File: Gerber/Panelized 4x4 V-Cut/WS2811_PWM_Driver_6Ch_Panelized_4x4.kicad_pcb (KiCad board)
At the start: 2 copper layers, 100 x 100 mm, 656 parts, among them P1 Com, P2 PWM, P3 HS/LS, P4 HS/LS, P5 GND, P6 DIFIN, P7 DIFOUT, Q1 MMBT4401, Q2 MMBT4401, Q3 MMBT4401, Q4 MMBT4401, Q5 MMBT4401, Q6 MMBT4401, U1 SP485, U2 WS2811, U3 WS2811, U4 SP485

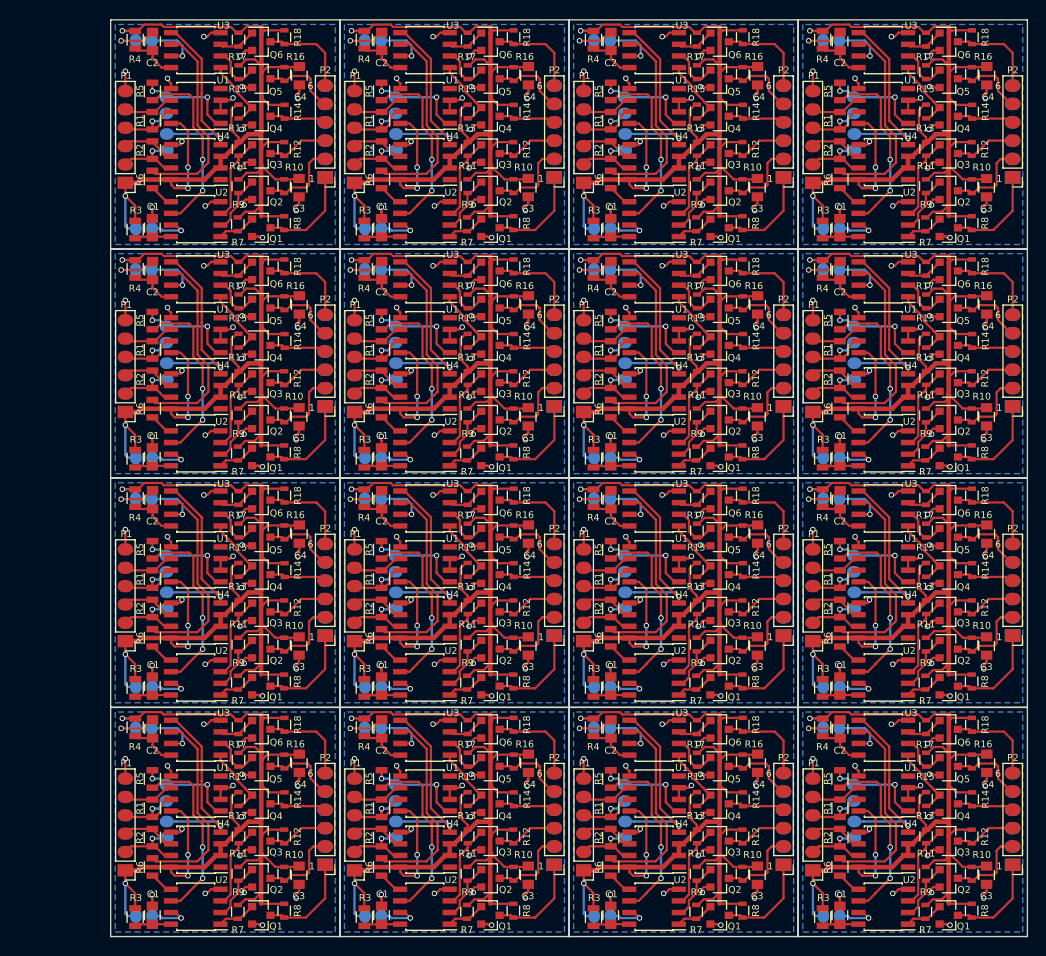
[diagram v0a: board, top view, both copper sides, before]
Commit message: Gerber Updates
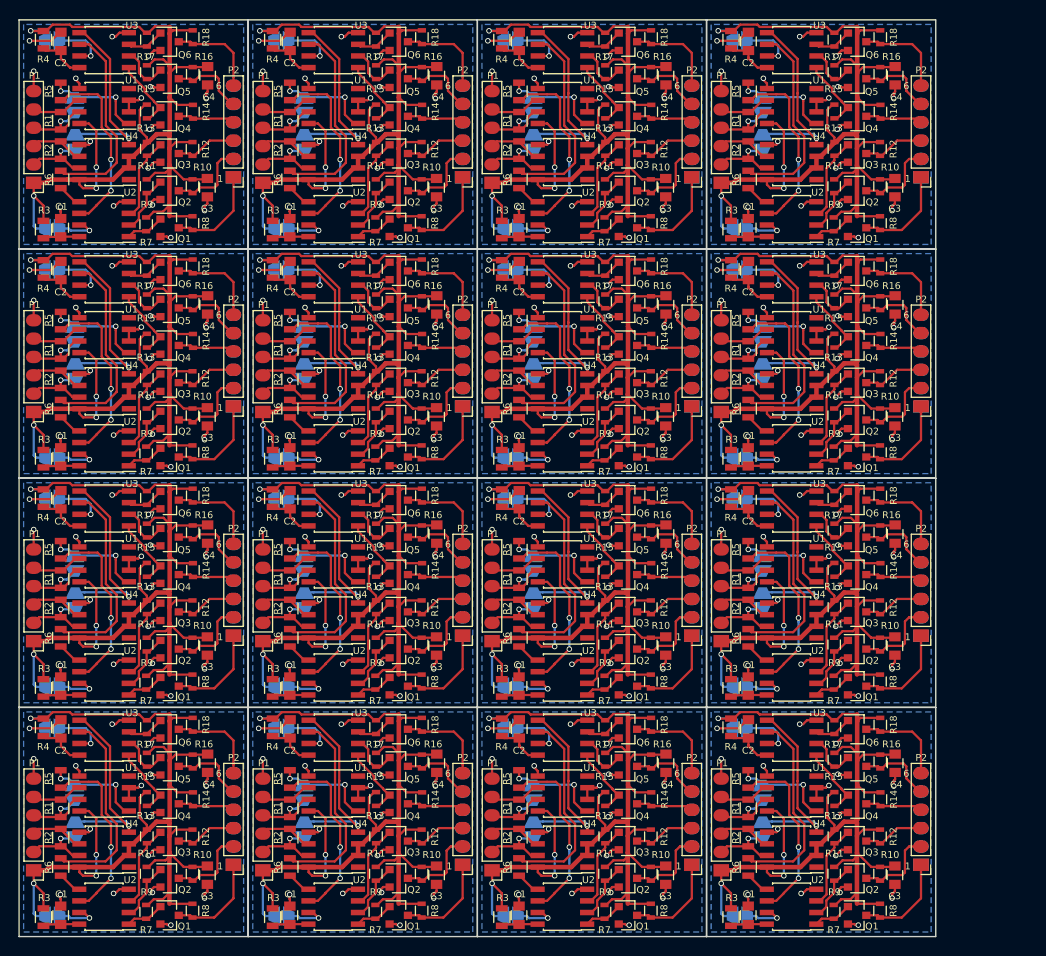
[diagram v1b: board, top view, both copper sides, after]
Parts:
- removed the C1 at (154.5, 147.7)
- removed the C1 at (129.5, 97.7)
- removed the C1 at (104.5, 97.7)
- removed the C1 at (179.5, 97.7)
- removed the C1 at (179.5, 72.7)
- removed the C1 at (154.5, 72.7)
- removed the C1 at (129.5, 72.7)
- removed the C1 at (129.5, 147.7)
- removed the C1 at (104.5, 147.7)
- removed the C1 at (179.5, 147.7)
- removed the C1 at (154.5, 122.7)
- removed the C1 at (129.5, 122.7)
- removed the C1 at (104.5, 122.7)
- removed the C1 at (179.5, 122.7)
- removed the C1 at (154.5, 97.7)
- removed the C2 at (154.6, 127.3)
- removed the C2 at (129.6, 77.3)
- removed the C2 at (104.6, 77.3)
- removed the C2 at (179.6, 77.3)
- removed the C2 at (179.6, 52.3)
- removed the C2 at (154.6, 52.3)
- removed the C2 at (129.6, 52.3)
- removed the C2 at (129.6, 127.3)
- removed the C2 at (104.6, 127.3)
- removed the C2 at (179.6, 127.3)
- removed the C2 at (154.6, 102.3)
- removed the C2 at (129.6, 102.3)
- removed the C2 at (104.6, 102.3)
- removed the C2 at (179.6, 102.3)
- removed the C2 at (154.6, 77.3)
- removed the C3 at (170.5, 143.3)
- removed the C3 at (145.5, 93.3)
- removed the C3 at (120.5, 93.3)
- removed the C3 at (195.5, 93.3)
- removed the C3 at (195.5, 68.3)
- removed the C3 at (170.5, 68.3)
- removed the C3 at (145.5, 68.3)
- removed the C3 at (145.5, 143.3)
- removed the C3 at (120.5, 143.3)
- removed the C3 at (195.5, 143.3)
- removed the C3 at (170.5, 118.3)
- removed the C3 at (145.5, 118.3)
- removed the C3 at (120.5, 118.3)
- removed the C3 at (195.5, 118.3)
- removed the C3 at (170.5, 93.3)
- removed the C4 at (170.6, 131.1)
- removed the C4 at (145.6, 81.1)
- removed the C4 at (120.6, 81.1)
- removed the C4 at (195.6, 81.1)
- removed the C4 at (195.6, 56.1)
- removed the C4 at (170.6, 56.1)
- removed the C4 at (145.6, 56.1)
- removed the C4 at (145.6, 131.1)
- removed the C4 at (120.6, 131.1)
- removed the C4 at (195.6, 131.1)
- removed the C4 at (170.6, 106.1)
- removed the C4 at (145.6, 106.1)
- removed the C4 at (120.6, 106.1)
- removed the C4 at (195.6, 106.1)
- removed the C4 at (170.6, 81.1)
- removed the P1 at (151.6, 142.8)
- removed the P1 at (126.6, 92.8)
- removed the P1 at (101.6, 92.8)
- removed the P1 at (176.6, 92.8)
- removed the P1 at (176.6, 67.8)
- removed the P1 at (151.6, 67.8)
- removed the P1 at (126.6, 67.8)
- removed the P1 at (126.6, 142.8)
- removed the P1 at (101.6, 142.8)
- removed the P1 at (176.6, 142.8)
- removed the P1 at (151.6, 117.8)
- removed the P1 at (126.6, 117.8)
- removed the P1 at (101.6, 117.8)
- removed the P1 at (176.6, 117.8)
- removed the P1 at (151.6, 92.8)
- removed the P2 at (148.4, 142.2)
- removed the P2 at (123.4, 92.2)
- removed the P2 at (173.4, 92.2)
- removed the P2 at (198.4, 92.2)
- removed the P2 at (198.4, 67.2)
- removed the P2 at (173.4, 67.2)
- removed the P2 at (148.4, 67.2)
- removed the P2 at (123.4, 142.2)
- removed the P2 at (173.4, 142.2)
- removed the P2 at (198.4, 142.2)
- removed the P2 at (148.4, 117.2)
- removed the P2 at (123.4, 117.2)
- removed the P2 at (173.4, 117.2)
- removed the P2 at (198.4, 117.2)
- removed the P2 at (148.4, 92.2)
- removed the P3 at (153.6, 147.8)
- removed the P3 at (178.6, 97.8)
- removed the P3 at (103.6, 97.8)
- removed the P3 at (128.6, 97.8)
- removed the P3 at (178.6, 72.8)
- removed the P3 at (153.6, 72.8)
- removed the P3 at (128.6, 72.8)
- removed the P3 at (178.6, 147.8)
- removed the P3 at (103.6, 147.8)
- removed the P3 at (128.6, 147.8)
- removed the P3 at (153.6, 122.8)
- removed the P3 at (178.6, 122.8)
- removed the P3 at (103.6, 122.8)
- removed the P3 at (128.6, 122.8)
- removed the P3 at (153.6, 97.8)
- removed the P4 at (153.6, 127.3)
- removed the P4 at (178.6, 77.3)
- removed the P4 at (103.6, 77.3)
- removed the P4 at (128.6, 77.3)
- removed the P4 at (178.6, 52.3)
- removed the P4 at (153.6, 52.3)
- removed the P4 at (128.6, 52.3)
- removed the P4 at (178.6, 127.3)
- removed the P4 at (103.6, 127.3)
- removed the P4 at (128.6, 127.3)
- removed the P4 at (153.6, 102.3)
- removed the P4 at (178.6, 102.3)
- removed the P4 at (103.6, 102.3)
- removed the P4 at (128.6, 102.3)
- removed the P4 at (153.6, 77.3)
- removed the P5 at (198.4, 142.2)
- removed the P5 at (148.4, 92.2)
- removed the P5 at (173.4, 92.2)
- removed the P5 at (123.4, 92.2)
- removed the P5 at (198.4, 67.2)
- removed the P5 at (173.4, 67.2)
- removed the P5 at (148.4, 67.2)
- removed the P5 at (148.4, 142.2)
- removed the P5 at (173.4, 142.2)
- removed the P5 at (123.4, 142.2)
- removed the P5 at (198.4, 117.2)
- removed the P5 at (148.4, 117.2)
- removed the P5 at (173.4, 117.2)
- removed the P5 at (123.4, 117.2)
- removed the P5 at (198.4, 92.2)
- removed the P6 at (181.1, 134.3)
- removed the P6 at (156.1, 84.3)
- removed the P6 at (106.1, 84.3)
- removed the P6 at (131.1, 84.3)
- removed the P6 at (181.1, 59.3)
- removed the P6 at (156.1, 59.3)
- removed the P6 at (131.1, 59.3)
- removed the P6 at (156.1, 134.3)
- removed the P6 at (106.1, 134.3)
- removed the P6 at (131.1, 134.3)
- removed the P6 at (181.1, 109.3)
- removed the P6 at (156.1, 109.3)
- removed the P6 at (106.1, 109.3)
- removed the P6 at (131.1, 109.3)
- removed the P6 at (181.1, 84.3)
- removed the P7 at (181.1, 138.3)
- removed the P7 at (156.1, 88.3)
- removed the P7 at (106.1, 88.3)
- removed the P7 at (131.1, 88.3)
- removed the P7 at (181.1, 63.3)
- removed the P7 at (156.1, 63.3)
- removed the P7 at (131.1, 63.3)
- removed the P7 at (156.1, 138.3)
- removed the P7 at (106.1, 138.3)
- removed the P7 at (131.1, 138.3)
- removed the P7 at (181.1, 113.3)
- removed the P7 at (156.1, 113.3)
- removed the P7 at (106.1, 113.3)
- removed the P7 at (131.1, 113.3)
- removed the P7 at (181.1, 88.3)
- removed the Q1 at (166.4, 147.7)
- removed the Q1 at (141.4, 97.7)
- removed the Q1 at (116.4, 97.7)
- removed the Q1 at (191.4, 97.7)
- removed the Q1 at (191.4, 72.7)
- removed the Q1 at (166.4, 72.7)
- removed the Q1 at (141.4, 72.7)
- removed the Q1 at (141.4, 147.7)
- removed the Q1 at (116.4, 147.7)
- removed the Q1 at (191.4, 147.7)
- removed the Q1 at (166.4, 122.7)
- removed the Q1 at (141.4, 122.7)
- removed the Q1 at (116.4, 122.7)
- removed the Q1 at (191.4, 122.7)
- removed the Q1 at (166.4, 97.7)
- removed the Q2 at (166.4, 143.6)
- removed the Q2 at (141.4, 93.6)
- removed the Q2 at (116.4, 93.6)
- removed the Q2 at (191.4, 93.6)
- removed the Q2 at (191.4, 68.6)
- removed the Q2 at (166.4, 68.6)
- removed the Q2 at (141.4, 68.6)
- removed the Q2 at (141.4, 143.6)
- removed the Q2 at (116.4, 143.6)
- removed the Q2 at (191.4, 143.6)
- removed the Q2 at (166.4, 118.6)
- removed the Q2 at (141.4, 118.6)
- removed the Q2 at (116.4, 118.6)
- removed the Q2 at (191.4, 118.6)
- removed the Q2 at (166.4, 93.6)
- removed the Q3 at (166.4, 139.6)
- removed the Q3 at (141.4, 89.6)
- removed the Q3 at (116.4, 89.6)
- removed the Q3 at (191.4, 89.6)
- removed the Q3 at (191.4, 64.6)
- removed the Q3 at (166.4, 64.6)
- removed the Q3 at (141.4, 64.6)
- removed the Q3 at (141.4, 139.6)
- removed the Q3 at (116.4, 139.6)
- removed the Q3 at (191.4, 139.6)
- removed the Q3 at (166.4, 114.6)
- removed the Q3 at (141.4, 114.6)
- removed the Q3 at (116.4, 114.6)
- removed the Q3 at (191.4, 114.6)
- removed the Q3 at (166.4, 89.6)
- removed the Q4 at (166.4, 135.5)
- removed the Q4 at (141.4, 85.5)
- removed the Q4 at (116.4, 85.5)
- removed the Q4 at (191.4, 85.5)
- removed the Q4 at (191.4, 60.5)
- removed the Q4 at (166.4, 60.5)
- removed the Q4 at (141.4, 60.5)
- removed the Q4 at (141.4, 135.5)
- removed the Q4 at (116.4, 135.5)
- removed the Q4 at (191.4, 135.5)
- removed the Q4 at (166.4, 110.5)
- removed the Q4 at (141.4, 110.5)
- removed the Q4 at (116.4, 110.5)
- removed the Q4 at (191.4, 110.5)
- removed the Q4 at (166.4, 85.5)
- removed the Q5 at (166.4, 131.4)
- removed the Q5 at (141.4, 81.4)
- removed the Q5 at (116.4, 81.4)
- removed the Q5 at (191.4, 81.4)
- removed the Q5 at (191.4, 56.4)
- removed the Q5 at (166.4, 56.4)
- removed the Q5 at (141.4, 56.4)
- removed the Q5 at (141.4, 131.4)
- removed the Q5 at (116.4, 131.4)
- removed the Q5 at (191.4, 131.4)
- removed the Q5 at (166.4, 106.4)
- removed the Q5 at (141.4, 106.4)
- removed the Q5 at (116.4, 106.4)
- removed the Q5 at (191.4, 106.4)
- removed the Q5 at (166.4, 81.4)
- removed the Q6 at (166.4, 127.4)
- removed the Q6 at (141.4, 77.4)
- removed the Q6 at (116.4, 77.4)
- removed the Q6 at (191.4, 77.4)
- removed the Q6 at (191.4, 52.4)
- removed the Q6 at (166.4, 52.4)
- removed the Q6 at (141.4, 52.4)
- removed the Q6 at (141.4, 127.4)
- removed the Q6 at (116.4, 127.4)
- removed the Q6 at (191.4, 127.4)
- removed the Q6 at (166.4, 102.4)
- removed the Q6 at (141.4, 102.4)
- removed the Q6 at (116.4, 102.4)
- removed the Q6 at (191.4, 102.4)
- removed the Q6 at (166.4, 77.4)
- removed the R1 at (154.5, 136.0)
- removed the R1 at (129.5, 86.0)
- removed the R1 at (104.5, 86.0)
- removed the R1 at (179.5, 86.0)
- removed the R1 at (179.5, 61.0)
- removed the R1 at (154.5, 61.0)
- removed the R1 at (129.5, 61.0)
- removed the R1 at (129.5, 136.0)
- removed the R1 at (104.5, 136.0)
- removed the R1 at (179.5, 136.0)
- removed the R1 at (154.5, 111.0)
- removed the R1 at (129.5, 111.0)
- removed the R1 at (104.5, 111.0)
- removed the R1 at (179.5, 111.0)
- removed the R1 at (154.5, 86.0)
- removed the R10 at (168.9, 143.1)
- removed the R10 at (143.9, 93.1)
- removed the R10 at (118.9, 93.1)
- removed the R10 at (193.9, 93.1)
- removed the R10 at (193.9, 68.1)
- removed the R10 at (168.9, 68.1)
- removed the R10 at (143.9, 68.1)
- removed the R10 at (143.9, 143.1)
- removed the R10 at (118.9, 143.1)
- removed the R10 at (193.9, 143.1)
- removed the R10 at (168.9, 118.1)
- removed the R10 at (143.9, 118.1)
- removed the R10 at (118.9, 118.1)
- removed the R10 at (193.9, 118.1)
- removed the R10 at (168.9, 93.1)
- removed the R11 at (163.9, 139.1)
- removed the R11 at (138.9, 89.1)
- removed the R11 at (113.9, 89.1)
- removed the R11 at (188.9, 89.1)
- removed the R11 at (188.9, 64.1)
- removed the R11 at (163.9, 64.1)
- removed the R11 at (138.9, 64.1)
- removed the R11 at (138.9, 139.1)
- removed the R11 at (113.9, 139.1)
- removed the R11 at (188.9, 139.1)
- removed the R11 at (163.9, 114.1)
- removed the R11 at (138.9, 114.1)
- removed the R11 at (113.9, 114.1)
- removed the R11 at (188.9, 114.1)
- removed the R11 at (163.9, 89.1)
- removed the R12 at (168.9, 139.1)
- removed the R12 at (143.9, 89.1)
- removed the R12 at (118.9, 89.1)
- removed the R12 at (193.9, 89.1)
- removed the R12 at (193.9, 64.1)
- removed the R12 at (168.9, 64.1)
- removed the R12 at (143.9, 64.1)
- removed the R12 at (143.9, 139.1)
- removed the R12 at (118.9, 139.1)
- removed the R12 at (193.9, 139.1)
- removed the R12 at (168.9, 114.1)
- removed the R12 at (143.9, 114.1)
- removed the R12 at (118.9, 114.1)
- removed the R12 at (193.9, 114.1)
- removed the R12 at (168.9, 89.1)
- removed the R13 at (163.9, 135.0)
- removed the R13 at (138.9, 85.0)
- removed the R13 at (113.9, 85.0)
- removed the R13 at (188.9, 85.0)
- removed the R13 at (188.9, 60.0)
- removed the R13 at (163.9, 60.0)
- removed the R13 at (138.9, 60.0)
- removed the R13 at (138.9, 135.0)
- removed the R13 at (113.9, 135.0)
- removed the R13 at (188.9, 135.0)
- removed the R13 at (163.9, 110.0)
- removed the R13 at (138.9, 110.0)
- removed the R13 at (113.9, 110.0)
- removed the R13 at (188.9, 110.0)
- removed the R13 at (163.9, 85.0)
- removed the R14 at (169.0, 135.0)
- removed the R14 at (144.0, 85.0)
- removed the R14 at (119.0, 85.0)
- removed the R14 at (194.0, 85.0)
- removed the R14 at (194.0, 60.0)
- removed the R14 at (169.0, 60.0)
- removed the R14 at (144.0, 60.0)
- removed the R14 at (144.0, 135.0)
- removed the R14 at (119.0, 135.0)
- removed the R14 at (194.0, 135.0)
- removed the R14 at (169.0, 110.0)
- removed the R14 at (144.0, 110.0)
- removed the R14 at (119.0, 110.0)
- removed the R14 at (194.0, 110.0)
- removed the R14 at (169.0, 85.0)
- removed the R15 at (163.9, 130.7)
- removed the R15 at (138.9, 80.7)
- removed the R15 at (113.9, 80.7)
- removed the R15 at (188.9, 80.7)
- removed the R15 at (188.9, 55.7)
- removed the R15 at (163.9, 55.7)
- removed the R15 at (138.9, 55.7)
- removed the R15 at (138.9, 130.7)
- removed the R15 at (113.9, 130.7)
- removed the R15 at (188.9, 130.7)
- removed the R15 at (163.9, 105.7)
- removed the R15 at (138.9, 105.7)
- removed the R15 at (113.9, 105.7)
- removed the R15 at (188.9, 105.7)
- removed the R15 at (163.9, 80.7)
- removed the R16 at (168.9, 130.9)
- removed the R16 at (143.9, 80.9)
- removed the R16 at (118.9, 80.9)
- removed the R16 at (193.9, 80.9)
- removed the R16 at (193.9, 55.9)
- removed the R16 at (168.9, 55.9)
- removed the R16 at (143.9, 55.9)
- removed the R16 at (143.9, 130.9)
- removed the R16 at (118.9, 130.9)
- removed the R16 at (193.9, 130.9)
- removed the R16 at (168.9, 105.9)
- removed the R16 at (143.9, 105.9)
- removed the R16 at (118.9, 105.9)
- removed the R16 at (193.9, 105.9)
- removed the R16 at (168.9, 80.9)
- removed the R17 at (163.9, 127.2)
- removed the R17 at (138.9, 77.2)
- removed the R17 at (113.9, 77.2)
- removed the R17 at (188.9, 77.2)
- removed the R17 at (188.9, 52.2)
- removed the R17 at (163.9, 52.2)
- removed the R17 at (138.9, 52.2)
- removed the R17 at (138.9, 127.2)
- removed the R17 at (113.9, 127.2)
- removed the R17 at (188.9, 127.2)
- removed the R17 at (163.9, 102.2)
- removed the R17 at (138.9, 102.2)
- removed the R17 at (113.9, 102.2)
- removed the R17 at (188.9, 102.2)
- removed the R17 at (163.9, 77.2)
- removed the R18 at (168.9, 126.9)
- removed the R18 at (143.9, 76.9)
- removed the R18 at (118.9, 76.9)
- removed the R18 at (193.9, 76.9)
- removed the R18 at (193.9, 51.9)
- removed the R18 at (168.9, 51.9)
- removed the R18 at (143.9, 51.9)
- removed the R18 at (143.9, 126.9)
- removed the R18 at (118.9, 126.9)
- removed the R18 at (193.9, 126.9)
- removed the R18 at (168.9, 101.9)
- removed the R18 at (143.9, 101.9)
- removed the R18 at (118.9, 101.9)
- removed the R18 at (193.9, 101.9)
- removed the R18 at (168.9, 76.9)
- removed the R2 at (154.5, 139.2)
- removed the R2 at (129.5, 89.2)
- removed the R2 at (104.5, 89.2)
- removed the R2 at (179.5, 89.2)
- removed the R2 at (179.5, 64.2)
- removed the R2 at (154.5, 64.2)
- removed the R2 at (129.5, 64.2)
- removed the R2 at (129.5, 139.2)
- removed the R2 at (104.5, 139.2)
- removed the R2 at (179.5, 139.2)
- removed the R2 at (154.5, 114.2)
- removed the R2 at (129.5, 114.2)
- removed the R2 at (104.5, 114.2)
- removed the R2 at (179.5, 114.2)
- removed the R2 at (154.5, 89.2)
- removed the R3 at (152.7, 147.9)
- removed the R3 at (127.7, 97.9)
- removed the R3 at (102.7, 97.9)
- removed the R3 at (177.7, 97.9)
- removed the R3 at (177.7, 72.9)
- removed the R3 at (152.7, 72.9)
- removed the R3 at (127.7, 72.9)
- removed the R3 at (127.7, 147.9)
- removed the R3 at (102.7, 147.9)
- removed the R3 at (177.7, 147.9)
- removed the R3 at (152.7, 122.9)
- removed the R3 at (127.7, 122.9)
- removed the R3 at (102.7, 122.9)
- removed the R3 at (177.7, 122.9)
- removed the R3 at (152.7, 97.9)
- removed the R4 at (152.7, 127.2)
- removed the R4 at (127.7, 77.2)
- removed the R4 at (102.7, 77.2)
- removed the R4 at (177.7, 77.2)
- removed the R4 at (177.7, 52.2)
- removed the R4 at (152.7, 52.2)
- removed the R4 at (127.7, 52.2)
- removed the R4 at (127.7, 127.2)
- removed the R4 at (102.7, 127.2)
- removed the R4 at (177.7, 127.2)
- removed the R4 at (152.7, 102.2)
- removed the R4 at (127.7, 102.2)
- removed the R4 at (102.7, 102.2)
- removed the R4 at (177.7, 102.2)
- removed the R4 at (152.7, 77.2)
- removed the R5 at (154.5, 132.8)
- removed the R5 at (129.5, 82.8)
- removed the R5 at (104.5, 82.8)
- removed the R5 at (179.5, 82.8)
- removed the R5 at (179.5, 57.8)
- removed the R5 at (154.5, 57.8)
- removed the R5 at (129.5, 57.8)
- removed the R5 at (129.5, 132.8)
- removed the R5 at (104.5, 132.8)
- removed the R5 at (179.5, 132.8)
- removed the R5 at (154.5, 107.8)
- removed the R5 at (129.5, 107.8)
- removed the R5 at (104.5, 107.8)
- removed the R5 at (179.5, 107.8)
- removed the R5 at (154.5, 82.8)
- removed the R6 at (154.5, 142.4)
- removed the R6 at (129.5, 92.4)
- removed the R6 at (104.5, 92.4)
- removed the R6 at (179.5, 92.4)
- removed the R6 at (179.5, 67.4)
- removed the R6 at (154.5, 67.4)
- removed the R6 at (129.5, 67.4)
- removed the R6 at (129.5, 142.4)
- removed the R6 at (104.5, 142.4)
- removed the R6 at (179.5, 142.4)
- removed the R6 at (154.5, 117.4)
- removed the R6 at (129.5, 117.4)
- removed the R6 at (104.5, 117.4)
- removed the R6 at (179.5, 117.4)
- removed the R6 at (154.5, 92.4)
- removed the R7 at (163.9, 147.3)
- removed the R7 at (138.9, 97.3)
- removed the R7 at (113.9, 97.3)
- removed the R7 at (188.9, 97.3)
- removed the R7 at (188.9, 72.3)
- removed the R7 at (163.9, 72.3)
- removed the R7 at (138.9, 72.3)
- removed the R7 at (138.9, 147.3)
- removed the R7 at (113.9, 147.3)
- removed the R7 at (188.9, 147.3)
- removed the R7 at (163.9, 122.3)
- removed the R7 at (138.9, 122.3)
- removed the R7 at (113.9, 122.3)
- removed the R7 at (188.9, 122.3)
- removed the R7 at (163.9, 97.3)
- removed the R8 at (168.9, 147.2)
- removed the R8 at (143.9, 97.2)
- removed the R8 at (118.9, 97.2)
- removed the R8 at (193.9, 97.2)
- removed the R8 at (193.9, 72.2)
- removed the R8 at (168.9, 72.2)
- removed the R8 at (143.9, 72.2)
- removed the R8 at (143.9, 147.2)
- removed the R8 at (118.9, 147.2)
- removed the R8 at (193.9, 147.2)
- removed the R8 at (168.9, 122.2)
- removed the R8 at (143.9, 122.2)
- removed the R8 at (118.9, 122.2)
- removed the R8 at (193.9, 122.2)
- removed the R8 at (168.9, 97.2)
- removed the R9 at (163.9, 143.1)
- removed the R9 at (138.9, 93.1)
- removed the R9 at (113.9, 93.1)
- removed the R9 at (188.9, 93.1)
- removed the R9 at (188.9, 68.1)
- removed the R9 at (163.9, 68.1)
- removed the R9 at (138.9, 68.1)
- removed the R9 at (138.9, 143.1)
- removed the R9 at (113.9, 143.1)
- removed the R9 at (188.9, 143.1)
- removed the R9 at (163.9, 118.1)
- removed the R9 at (138.9, 118.1)
- removed the R9 at (113.9, 118.1)
- removed the R9 at (188.9, 118.1)
- removed the R9 at (163.9, 93.1)
- removed the REF*** at (194.1, 139.9)
- removed the REF*** at (190.4, 121.3)
- removed the REF*** at (140.4, 121.3)
- removed the REF*** at (144.1, 114.9)
- removed the REF*** at (169.1, 114.9)
- removed the REF*** at (165.4, 121.3)
- removed the REF*** at (115.4, 121.3)
- removed the REF*** at (119.1, 114.9)
- removed the REF*** at (194.1, 89.9)
- removed the REF*** at (190.4, 96.3)
- removed the REF*** at (140.4, 96.3)
- removed the REF*** at (190.4, 146.3)
- removed the REF*** at (144.1, 89.9)
- removed the REF*** at (169.1, 89.9)
- removed the REF*** at (165.4, 96.3)
- removed the REF*** at (115.4, 96.3)
- removed the REF*** at (119.1, 89.9)
- removed the REF*** at (194.1, 64.9)
- removed the REF*** at (190.4, 71.3)
- removed the REF*** at (169.1, 64.9)
- removed the REF*** at (165.4, 71.3)
- removed the REF*** at (144.1, 64.9)
- removed the REF*** at (140.4, 146.3)
- removed the REF*** at (140.4, 71.3)
- removed the REF*** at (144.1, 139.9)
- removed the REF*** at (169.1, 139.9)
- removed the REF*** at (165.4, 146.3)
- removed the REF*** at (115.4, 146.3)
- removed the REF*** at (119.1, 139.9)
- removed the REF*** at (194.1, 114.9)
- removed the U1 at (159.3, 134.4)
- removed the U1 at (134.3, 84.4)
- removed the U1 at (109.3, 84.4)
- removed the U1 at (184.3, 84.4)
- removed the U1 at (184.3, 59.4)
- removed the U1 at (159.3, 59.4)
- removed the U1 at (134.3, 59.4)
- removed the U1 at (134.3, 134.4)
- removed the U1 at (109.3, 134.4)
- removed the U1 at (184.3, 134.4)
- removed the U1 at (159.3, 109.4)
- removed the U1 at (134.3, 109.4)
- removed the U1 at (109.3, 109.4)
- removed the U1 at (184.3, 109.4)
- removed the U1 at (159.3, 84.4)
- removed the U2 at (159.3, 146.7)
- removed the U2 at (134.3, 96.7)
- removed the U2 at (109.3, 96.7)
- removed the U2 at (184.3, 96.7)
- removed the U2 at (184.3, 71.7)
- removed the U2 at (159.3, 71.7)
- removed the U2 at (134.3, 71.7)
- removed the U2 at (134.3, 146.7)
- removed the U2 at (109.3, 146.7)
- removed the U2 at (184.3, 146.7)
- removed the U2 at (159.3, 121.7)
- removed the U2 at (134.3, 121.7)
- removed the U2 at (109.3, 121.7)
- removed the U2 at (184.3, 121.7)
- removed the U2 at (159.3, 96.7)
- removed the U3 at (159.3, 128.3)
- removed the U3 at (134.3, 78.3)
- removed the U3 at (109.3, 78.3)
- removed the U3 at (184.3, 78.3)
- removed the U3 at (184.3, 53.3)
- removed the U3 at (159.3, 53.3)
- removed the U3 at (134.3, 53.3)
- removed the U3 at (134.3, 128.3)
- removed the U3 at (109.3, 128.3)
- removed the U3 at (184.3, 128.3)
- removed the U3 at (159.3, 103.3)
- removed the U3 at (134.3, 103.3)
- removed the U3 at (109.3, 103.3)
- removed the U3 at (184.3, 103.3)
- removed the U3 at (159.3, 78.3)
- removed the U4 at (159.3, 140.5)
- removed the U4 at (134.3, 90.5)
- removed the U4 at (109.3, 90.5)
- removed the U4 at (184.3, 90.5)
- removed the U4 at (184.3, 65.5)
- removed the U4 at (159.3, 65.5)
- removed the U4 at (134.3, 65.5)
- removed the U4 at (134.3, 140.5)
- removed the U4 at (109.3, 140.5)
- removed the U4 at (184.3, 140.5)
- removed the U4 at (159.3, 115.5)
- removed the U4 at (134.3, 115.5)
- removed the U4 at (109.3, 115.5)
- removed the U4 at (184.3, 115.5)
- removed the U4 at (159.3, 90.5)
- added C1: 10n, Capacitors_SMD:C_0805, F.Cu at (169.5, 147.7)
- added C1: 10n, Capacitors_SMD:C_0805, F.Cu at (144.5, 97.7)
- added C1: 10n, Capacitors_SMD:C_0805, F.Cu at (119.5, 97.7)
- added C1: 10n, Capacitors_SMD:C_0805, F.Cu at (94.5, 97.7)
- added C1: 10n, Capacitors_SMD:C_0805, F.Cu at (169.5, 72.7)
- added C1: 10n, Capacitors_SMD:C_0805, F.Cu at (144.5, 72.7)
- added C1: 10n, Capacitors_SMD:C_0805, F.Cu at (119.5, 72.7)
- added C1: 10n, Capacitors_SMD:C_0805, F.Cu at (144.5, 147.7)
- added C1: 10n, Capacitors_SMD:C_0805, F.Cu at (119.5, 147.7)
- added C1: 10n, Capacitors_SMD:C_0805, F.Cu at (94.5, 147.7)
- added C1: 10n, Capacitors_SMD:C_0805, F.Cu at (169.5, 122.7)
- added C1: 10n, Capacitors_SMD:C_0805, F.Cu at (144.5, 122.7)
- added C1: 10n, Capacitors_SMD:C_0805, F.Cu at (119.5, 122.7)
- added C1: 10n, Capacitors_SMD:C_0805, F.Cu at (94.5, 122.7)
- added C1: 10n, Capacitors_SMD:C_0805, F.Cu at (169.5, 97.7)
- added C2: 10n, Capacitors_SMD:C_0805, F.Cu at (169.6, 127.3)
- added C2: 10n, Capacitors_SMD:C_0805, F.Cu at (144.6, 77.3)
- added C2: 10n, Capacitors_SMD:C_0805, F.Cu at (119.6, 77.3)
- added C2: 10n, Capacitors_SMD:C_0805, F.Cu at (94.6, 77.3)
- added C2: 10n, Capacitors_SMD:C_0805, F.Cu at (169.6, 52.3)
- added C2: 10n, Capacitors_SMD:C_0805, F.Cu at (144.6, 52.3)
- added C2: 10n, Capacitors_SMD:C_0805, F.Cu at (119.6, 52.3)
- added C2: 10n, Capacitors_SMD:C_0805, F.Cu at (144.6, 127.3)
- added C2: 10n, Capacitors_SMD:C_0805, F.Cu at (119.6, 127.3)
- added C2: 10n, Capacitors_SMD:C_0805, F.Cu at (94.6, 127.3)
- added C2: 10n, Capacitors_SMD:C_0805, F.Cu at (169.6, 102.3)
- added C2: 10n, Capacitors_SMD:C_0805, F.Cu at (144.6, 102.3)
- added C2: 10n, Capacitors_SMD:C_0805, F.Cu at (119.6, 102.3)
- added C2: 10n, Capacitors_SMD:C_0805, F.Cu at (94.6, 102.3)
- added C2: 10n, Capacitors_SMD:C_0805, F.Cu at (169.6, 77.3)
- added C3: 10u/10V, Capacitors_SMD:C_0805, F.Cu at (160.5, 143.3)
- added C3: 10u/10V, Capacitors_SMD:C_0805, F.Cu at (185.5, 93.3)
- added C3: 10u/10V, Capacitors_SMD:C_0805, F.Cu at (135.5, 93.3)
- added C3: 10u/10V, Capacitors_SMD:C_0805, F.Cu at (110.5, 93.3)
- added C3: 10u/10V, Capacitors_SMD:C_0805, F.Cu at (185.5, 68.3)
- added C3: 10u/10V, Capacitors_SMD:C_0805, F.Cu at (160.5, 68.3)
- added C3: 10u/10V, Capacitors_SMD:C_0805, F.Cu at (135.5, 68.3)
- added C3: 10u/10V, Capacitors_SMD:C_0805, F.Cu at (185.5, 143.3)
- added C3: 10u/10V, Capacitors_SMD:C_0805, F.Cu at (135.5, 143.3)
- added C3: 10u/10V, Capacitors_SMD:C_0805, F.Cu at (110.5, 143.3)
- added C3: 10u/10V, Capacitors_SMD:C_0805, F.Cu at (160.5, 118.3)
- added C3: 10u/10V, Capacitors_SMD:C_0805, F.Cu at (185.5, 118.3)
- added C3: 10u/10V, Capacitors_SMD:C_0805, F.Cu at (135.5, 118.3)
- added C3: 10u/10V, Capacitors_SMD:C_0805, F.Cu at (110.5, 118.3)
- added C3: 10u/10V, Capacitors_SMD:C_0805, F.Cu at (160.5, 93.3)
- added C4: 10u/10V, Capacitors_SMD:C_0805, F.Cu at (160.6, 131.1)
- added C4: 10u/10V, Capacitors_SMD:C_0805, F.Cu at (185.6, 81.1)
- added C4: 10u/10V, Capacitors_SMD:C_0805, F.Cu at (135.6, 81.1)
- added C4: 10u/10V, Capacitors_SMD:C_0805, F.Cu at (110.6, 81.1)
- added C4: 10u/10V, Capacitors_SMD:C_0805, F.Cu at (185.6, 56.1)
- added C4: 10u/10V, Capacitors_SMD:C_0805, F.Cu at (160.6, 56.1)
- added C4: 10u/10V, Capacitors_SMD:C_0805, F.Cu at (135.6, 56.1)
- added C4: 10u/10V, Capacitors_SMD:C_0805, F.Cu at (185.6, 131.1)
- added C4: 10u/10V, Capacitors_SMD:C_0805, F.Cu at (135.6, 131.1)
- added C4: 10u/10V, Capacitors_SMD:C_0805, F.Cu at (110.6, 131.1)
- added C4: 10u/10V, Capacitors_SMD:C_0805, F.Cu at (160.6, 106.1)
- added C4: 10u/10V, Capacitors_SMD:C_0805, F.Cu at (185.6, 106.1)
- added C4: 10u/10V, Capacitors_SMD:C_0805, F.Cu at (135.6, 106.1)
- added C4: 10u/10V, Capacitors_SMD:C_0805, F.Cu at (110.6, 106.1)
- added C4: 10u/10V, Capacitors_SMD:C_0805, F.Cu at (160.6, 81.1)
- added P1: Com, PCB FootPrints:Pin_Header_Straight_1x06_Pitch2.00mm, F.Cu at (166.6, 142.8)
- added P1: Com, PCB FootPrints:Pin_Header_Straight_1x06_Pitch2.00mm, F.Cu at (141.6, 92.8)
- added P1: Com, PCB FootPrints:Pin_Header_Straight_1x06_Pitch2.00mm, F.Cu at (116.6, 92.8)
- added P1: Com, PCB FootPrints:Pin_Header_Straight_1x06_Pitch2.00mm, F.Cu at (91.6, 92.8)
- added P1: Com, PCB FootPrints:Pin_Header_Straight_1x06_Pitch2.00mm, F.Cu at (166.6, 67.8)
- added P1: Com, PCB FootPrints:Pin_Header_Straight_1x06_Pitch2.00mm, F.Cu at (141.6, 67.8)
- added P1: Com, PCB FootPrints:Pin_Header_Straight_1x06_Pitch2.00mm, F.Cu at (116.6, 67.8)
- added P1: Com, PCB FootPrints:Pin_Header_Straight_1x06_Pitch2.00mm, F.Cu at (141.6, 142.8)
- added P1: Com, PCB FootPrints:Pin_Header_Straight_1x06_Pitch2.00mm, F.Cu at (116.6, 142.8)
- added P1: Com, PCB FootPrints:Pin_Header_Straight_1x06_Pitch2.00mm, F.Cu at (91.6, 142.8)
- added P1: Com, PCB FootPrints:Pin_Header_Straight_1x06_Pitch2.00mm, F.Cu at (166.6, 117.8)
- added P1: Com, PCB FootPrints:Pin_Header_Straight_1x06_Pitch2.00mm, F.Cu at (141.6, 117.8)
- added P1: Com, PCB FootPrints:Pin_Header_Straight_1x06_Pitch2.00mm, F.Cu at (116.6, 117.8)
- added P1: Com, PCB FootPrints:Pin_Header_Straight_1x06_Pitch2.00mm, F.Cu at (91.6, 117.8)
- added P1: Com, PCB FootPrints:Pin_Header_Straight_1x06_Pitch2.00mm, F.Cu at (166.6, 92.8)
- added P2: PWM, PCB FootPrints:Pin_Header_Straight_1x06_Pitch2.00mm, F.Cu at (163.4, 142.2)
- added P2: PWM, PCB FootPrints:Pin_Header_Straight_1x06_Pitch2.00mm, F.Cu at (188.4, 92.2)
- added P2: PWM, PCB FootPrints:Pin_Header_Straight_1x06_Pitch2.00mm, F.Cu at (138.4, 92.2)
- added P2: PWM, PCB FootPrints:Pin_Header_Straight_1x06_Pitch2.00mm, F.Cu at (113.4, 92.2)
- added P2: PWM, PCB FootPrints:Pin_Header_Straight_1x06_Pitch2.00mm, F.Cu at (188.4, 67.2)
- added P2: PWM, PCB FootPrints:Pin_Header_Straight_1x06_Pitch2.00mm, F.Cu at (163.4, 67.2)
- added P2: PWM, PCB FootPrints:Pin_Header_Straight_1x06_Pitch2.00mm, F.Cu at (138.4, 67.2)
- added P2: PWM, PCB FootPrints:Pin_Header_Straight_1x06_Pitch2.00mm, F.Cu at (188.4, 142.2)
- added P2: PWM, PCB FootPrints:Pin_Header_Straight_1x06_Pitch2.00mm, F.Cu at (138.4, 142.2)
- added P2: PWM, PCB FootPrints:Pin_Header_Straight_1x06_Pitch2.00mm, F.Cu at (113.4, 142.2)
- added P2: PWM, PCB FootPrints:Pin_Header_Straight_1x06_Pitch2.00mm, F.Cu at (163.4, 117.2)
- added P2: PWM, PCB FootPrints:Pin_Header_Straight_1x06_Pitch2.00mm, F.Cu at (188.4, 117.2)
- added P2: PWM, PCB FootPrints:Pin_Header_Straight_1x06_Pitch2.00mm, F.Cu at (138.4, 117.2)
- added P2: PWM, PCB FootPrints:Pin_Header_Straight_1x06_Pitch2.00mm, F.Cu at (113.4, 117.2)
- added P2: PWM, PCB FootPrints:Pin_Header_Straight_1x06_Pitch2.00mm, F.Cu at (163.4, 92.2)
- added P3: HS/LS, BK_Common:2_pin_solder_jumper_smd, B.Cu at (168.6, 147.8)
- added P3: HS/LS, BK_Common:2_pin_solder_jumper_smd, B.Cu at (143.6, 97.8)
- added P3: HS/LS, BK_Common:2_pin_solder_jumper_smd, B.Cu at (93.6, 97.8)
- added P3: HS/LS, BK_Common:2_pin_solder_jumper_smd, B.Cu at (118.6, 97.8)
- added P3: HS/LS, BK_Common:2_pin_solder_jumper_smd, B.Cu at (143.6, 72.8)
- added P3: HS/LS, BK_Common:2_pin_solder_jumper_smd, B.Cu at (168.6, 72.8)
- added P3: HS/LS, BK_Common:2_pin_solder_jumper_smd, B.Cu at (118.6, 72.8)
- added P3: HS/LS, BK_Common:2_pin_solder_jumper_smd, B.Cu at (143.6, 147.8)
- added P3: HS/LS, BK_Common:2_pin_solder_jumper_smd, B.Cu at (93.6, 147.8)
- added P3: HS/LS, BK_Common:2_pin_solder_jumper_smd, B.Cu at (118.6, 147.8)
- added P3: HS/LS, BK_Common:2_pin_solder_jumper_smd, B.Cu at (168.6, 122.8)
- added P3: HS/LS, BK_Common:2_pin_solder_jumper_smd, B.Cu at (143.6, 122.8)
- added P3: HS/LS, BK_Common:2_pin_solder_jumper_smd, B.Cu at (93.6, 122.8)
- added P3: HS/LS, BK_Common:2_pin_solder_jumper_smd, B.Cu at (118.6, 122.8)
- added P3: HS/LS, BK_Common:2_pin_solder_jumper_smd, B.Cu at (168.6, 97.8)
- added P4: HS/LS, BK_Common:2_pin_solder_jumper_smd, B.Cu at (168.6, 127.3)
- added P4: HS/LS, BK_Common:2_pin_solder_jumper_smd, B.Cu at (143.6, 77.3)
- added P4: HS/LS, BK_Common:2_pin_solder_jumper_smd, B.Cu at (93.6, 77.3)
- added P4: HS/LS, BK_Common:2_pin_solder_jumper_smd, B.Cu at (118.6, 77.3)
- added P4: HS/LS, BK_Common:2_pin_solder_jumper_smd, B.Cu at (143.6, 52.3)
- added P4: HS/LS, BK_Common:2_pin_solder_jumper_smd, B.Cu at (168.6, 52.3)
- added P4: HS/LS, BK_Common:2_pin_solder_jumper_smd, B.Cu at (118.6, 52.3)
- added P4: HS/LS, BK_Common:2_pin_solder_jumper_smd, B.Cu at (143.6, 127.3)
- added P4: HS/LS, BK_Common:2_pin_solder_jumper_smd, B.Cu at (93.6, 127.3)
- added P4: HS/LS, BK_Common:2_pin_solder_jumper_smd, B.Cu at (118.6, 127.3)
- added P4: HS/LS, BK_Common:2_pin_solder_jumper_smd, B.Cu at (168.6, 102.3)
- added P4: HS/LS, BK_Common:2_pin_solder_jumper_smd, B.Cu at (143.6, 102.3)
- added P4: HS/LS, BK_Common:2_pin_solder_jumper_smd, B.Cu at (93.6, 102.3)
- added P4: HS/LS, BK_Common:2_pin_solder_jumper_smd, B.Cu at (118.6, 102.3)
- added P4: HS/LS, BK_Common:2_pin_solder_jumper_smd, B.Cu at (168.6, 77.3)
- added P5: GND, PCB FootPrints:Pin_Header_Straight_1x06_Pitch2.00mm, B.Cu at (163.4, 142.2)
- added P5: GND, PCB FootPrints:Pin_Header_Straight_1x06_Pitch2.00mm, B.Cu at (138.4, 92.2)
- added P5: GND, PCB FootPrints:Pin_Header_Straight_1x06_Pitch2.00mm, B.Cu at (188.4, 92.2)
- added P5: GND, PCB FootPrints:Pin_Header_Straight_1x06_Pitch2.00mm, B.Cu at (113.4, 92.2)
- added P5: GND, PCB FootPrints:Pin_Header_Straight_1x06_Pitch2.00mm, B.Cu at (163.4, 67.2)
- added P5: GND, PCB FootPrints:Pin_Header_Straight_1x06_Pitch2.00mm, B.Cu at (188.4, 67.2)
- added P5: GND, PCB FootPrints:Pin_Header_Straight_1x06_Pitch2.00mm, B.Cu at (138.4, 67.2)
- added P5: GND, PCB FootPrints:Pin_Header_Straight_1x06_Pitch2.00mm, B.Cu at (138.4, 142.2)
- added P5: GND, PCB FootPrints:Pin_Header_Straight_1x06_Pitch2.00mm, B.Cu at (188.4, 142.2)
- added P5: GND, PCB FootPrints:Pin_Header_Straight_1x06_Pitch2.00mm, B.Cu at (113.4, 142.2)
- added P5: GND, PCB FootPrints:Pin_Header_Straight_1x06_Pitch2.00mm, B.Cu at (163.4, 117.2)
- added P5: GND, PCB FootPrints:Pin_Header_Straight_1x06_Pitch2.00mm, B.Cu at (138.4, 117.2)
- added P5: GND, PCB FootPrints:Pin_Header_Straight_1x06_Pitch2.00mm, B.Cu at (188.4, 117.2)
- added P5: GND, PCB FootPrints:Pin_Header_Straight_1x06_Pitch2.00mm, B.Cu at (113.4, 117.2)
- added P5: GND, PCB FootPrints:Pin_Header_Straight_1x06_Pitch2.00mm, B.Cu at (163.4, 92.2)
- added P6: DIFIN, BK_Common:2_pin_solder_jumper_smd, B.Cu at (146.1, 134.3)
- added P6: DIFIN, BK_Common:2_pin_solder_jumper_smd, B.Cu at (171.1, 84.3)
- added P6: DIFIN, BK_Common:2_pin_solder_jumper_smd, B.Cu at (96.1, 84.3)
- added P6: DIFIN, BK_Common:2_pin_solder_jumper_smd, B.Cu at (121.1, 84.3)
- added P6: DIFIN, BK_Common:2_pin_solder_jumper_smd, B.Cu at (146.1, 59.3)
- added P6: DIFIN, BK_Common:2_pin_solder_jumper_smd, B.Cu at (171.1, 59.3)
- added P6: DIFIN, BK_Common:2_pin_solder_jumper_smd, B.Cu at (121.1, 59.3)
- added P6: DIFIN, BK_Common:2_pin_solder_jumper_smd, B.Cu at (171.1, 134.3)
- added P6: DIFIN, BK_Common:2_pin_solder_jumper_smd, B.Cu at (96.1, 134.3)
- added P6: DIFIN, BK_Common:2_pin_solder_jumper_smd, B.Cu at (121.1, 134.3)
- added P6: DIFIN, BK_Common:2_pin_solder_jumper_smd, B.Cu at (146.1, 109.3)
- added P6: DIFIN, BK_Common:2_pin_solder_jumper_smd, B.Cu at (171.1, 109.3)
- added P6: DIFIN, BK_Common:2_pin_solder_jumper_smd, B.Cu at (96.1, 109.3)
- added P6: DIFIN, BK_Common:2_pin_solder_jumper_smd, B.Cu at (121.1, 109.3)
- added P6: DIFIN, BK_Common:2_pin_solder_jumper_smd, B.Cu at (146.1, 84.3)
- added P7: DIFOUT, BK_Common:2_pin_solder_jumper_smd, B.Cu at (146.1, 138.3)
- added P7: DIFOUT, BK_Common:2_pin_solder_jumper_smd, B.Cu at (171.1, 88.3)
- added P7: DIFOUT, BK_Common:2_pin_solder_jumper_smd, B.Cu at (96.1, 88.3)
- added P7: DIFOUT, BK_Common:2_pin_solder_jumper_smd, B.Cu at (121.1, 88.3)
- added P7: DIFOUT, BK_Common:2_pin_solder_jumper_smd, B.Cu at (146.1, 63.3)
- added P7: DIFOUT, BK_Common:2_pin_solder_jumper_smd, B.Cu at (171.1, 63.3)
- added P7: DIFOUT, BK_Common:2_pin_solder_jumper_smd, B.Cu at (121.1, 63.3)
- added P7: DIFOUT, BK_Common:2_pin_solder_jumper_smd, B.Cu at (171.1, 138.3)
- added P7: DIFOUT, BK_Common:2_pin_solder_jumper_smd, B.Cu at (96.1, 138.3)
- added P7: DIFOUT, BK_Common:2_pin_solder_jumper_smd, B.Cu at (121.1, 138.3)
- added P7: DIFOUT, BK_Common:2_pin_solder_jumper_smd, B.Cu at (146.1, 113.3)
- added P7: DIFOUT, BK_Common:2_pin_solder_jumper_smd, B.Cu at (171.1, 113.3)
- added P7: DIFOUT, BK_Common:2_pin_solder_jumper_smd, B.Cu at (96.1, 113.3)
- added P7: DIFOUT, BK_Common:2_pin_solder_jumper_smd, B.Cu at (121.1, 113.3)
- added P7: DIFOUT, BK_Common:2_pin_solder_jumper_smd, B.Cu at (146.1, 88.3)
- added Q1: MMBT4401, WS2811_PWM_PCB:SOT-23, F.Cu at (156.4, 147.7)
- added Q1: MMBT4401, WS2811_PWM_PCB:SOT-23, F.Cu at (181.4, 97.7)
- added Q1: MMBT4401, WS2811_PWM_PCB:SOT-23, F.Cu at (131.4, 97.7)
- added Q1: MMBT4401, WS2811_PWM_PCB:SOT-23, F.Cu at (106.4, 97.7)
- added Q1: MMBT4401, WS2811_PWM_PCB:SOT-23, F.Cu at (181.4, 72.7)
- added Q1: MMBT4401, WS2811_PWM_PCB:SOT-23, F.Cu at (156.4, 72.7)
- added Q1: MMBT4401, WS2811_PWM_PCB:SOT-23, F.Cu at (131.4, 72.7)
- added Q1: MMBT4401, WS2811_PWM_PCB:SOT-23, F.Cu at (181.4, 147.7)
- added Q1: MMBT4401, WS2811_PWM_PCB:SOT-23, F.Cu at (131.4, 147.7)
- added Q1: MMBT4401, WS2811_PWM_PCB:SOT-23, F.Cu at (106.4, 147.7)
- added Q1: MMBT4401, WS2811_PWM_PCB:SOT-23, F.Cu at (156.4, 122.7)
- added Q1: MMBT4401, WS2811_PWM_PCB:SOT-23, F.Cu at (181.4, 122.7)
- added Q1: MMBT4401, WS2811_PWM_PCB:SOT-23, F.Cu at (131.4, 122.7)
- added Q1: MMBT4401, WS2811_PWM_PCB:SOT-23, F.Cu at (106.4, 122.7)
- added Q1: MMBT4401, WS2811_PWM_PCB:SOT-23, F.Cu at (156.4, 97.7)
- added Q2: MMBT4401, WS2811_PWM_PCB:SOT-23, F.Cu at (156.4, 143.6)
- added Q2: MMBT4401, WS2811_PWM_PCB:SOT-23, F.Cu at (181.4, 93.6)
- added Q2: MMBT4401, WS2811_PWM_PCB:SOT-23, F.Cu at (131.4, 93.6)
- added Q2: MMBT4401, WS2811_PWM_PCB:SOT-23, F.Cu at (106.4, 93.6)
- added Q2: MMBT4401, WS2811_PWM_PCB:SOT-23, F.Cu at (181.4, 68.6)
- added Q2: MMBT4401, WS2811_PWM_PCB:SOT-23, F.Cu at (156.4, 68.6)
- added Q2: MMBT4401, WS2811_PWM_PCB:SOT-23, F.Cu at (131.4, 68.6)
- added Q2: MMBT4401, WS2811_PWM_PCB:SOT-23, F.Cu at (181.4, 143.6)
- added Q2: MMBT4401, WS2811_PWM_PCB:SOT-23, F.Cu at (131.4, 143.6)
- added Q2: MMBT4401, WS2811_PWM_PCB:SOT-23, F.Cu at (106.4, 143.6)
- added Q2: MMBT4401, WS2811_PWM_PCB:SOT-23, F.Cu at (156.4, 118.6)
- added Q2: MMBT4401, WS2811_PWM_PCB:SOT-23, F.Cu at (181.4, 118.6)
- added Q2: MMBT4401, WS2811_PWM_PCB:SOT-23, F.Cu at (131.4, 118.6)
- added Q2: MMBT4401, WS2811_PWM_PCB:SOT-23, F.Cu at (106.4, 118.6)
- added Q2: MMBT4401, WS2811_PWM_PCB:SOT-23, F.Cu at (156.4, 93.6)
- added Q3: MMBT4401, WS2811_PWM_PCB:SOT-23, F.Cu at (156.4, 139.6)
- added Q3: MMBT4401, WS2811_PWM_PCB:SOT-23, F.Cu at (181.4, 89.6)
- added Q3: MMBT4401, WS2811_PWM_PCB:SOT-23, F.Cu at (131.4, 89.6)
- added Q3: MMBT4401, WS2811_PWM_PCB:SOT-23, F.Cu at (106.4, 89.6)
- added Q3: MMBT4401, WS2811_PWM_PCB:SOT-23, F.Cu at (181.4, 64.6)
- added Q3: MMBT4401, WS2811_PWM_PCB:SOT-23, F.Cu at (156.4, 64.6)
- added Q3: MMBT4401, WS2811_PWM_PCB:SOT-23, F.Cu at (131.4, 64.6)
- added Q3: MMBT4401, WS2811_PWM_PCB:SOT-23, F.Cu at (181.4, 139.6)
- added Q3: MMBT4401, WS2811_PWM_PCB:SOT-23, F.Cu at (131.4, 139.6)
- added Q3: MMBT4401, WS2811_PWM_PCB:SOT-23, F.Cu at (106.4, 139.6)
- added Q3: MMBT4401, WS2811_PWM_PCB:SOT-23, F.Cu at (156.4, 114.6)
- added Q3: MMBT4401, WS2811_PWM_PCB:SOT-23, F.Cu at (181.4, 114.6)
- added Q3: MMBT4401, WS2811_PWM_PCB:SOT-23, F.Cu at (131.4, 114.6)
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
